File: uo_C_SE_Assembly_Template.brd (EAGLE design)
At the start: 40 x 110.5 mm, 0 parts

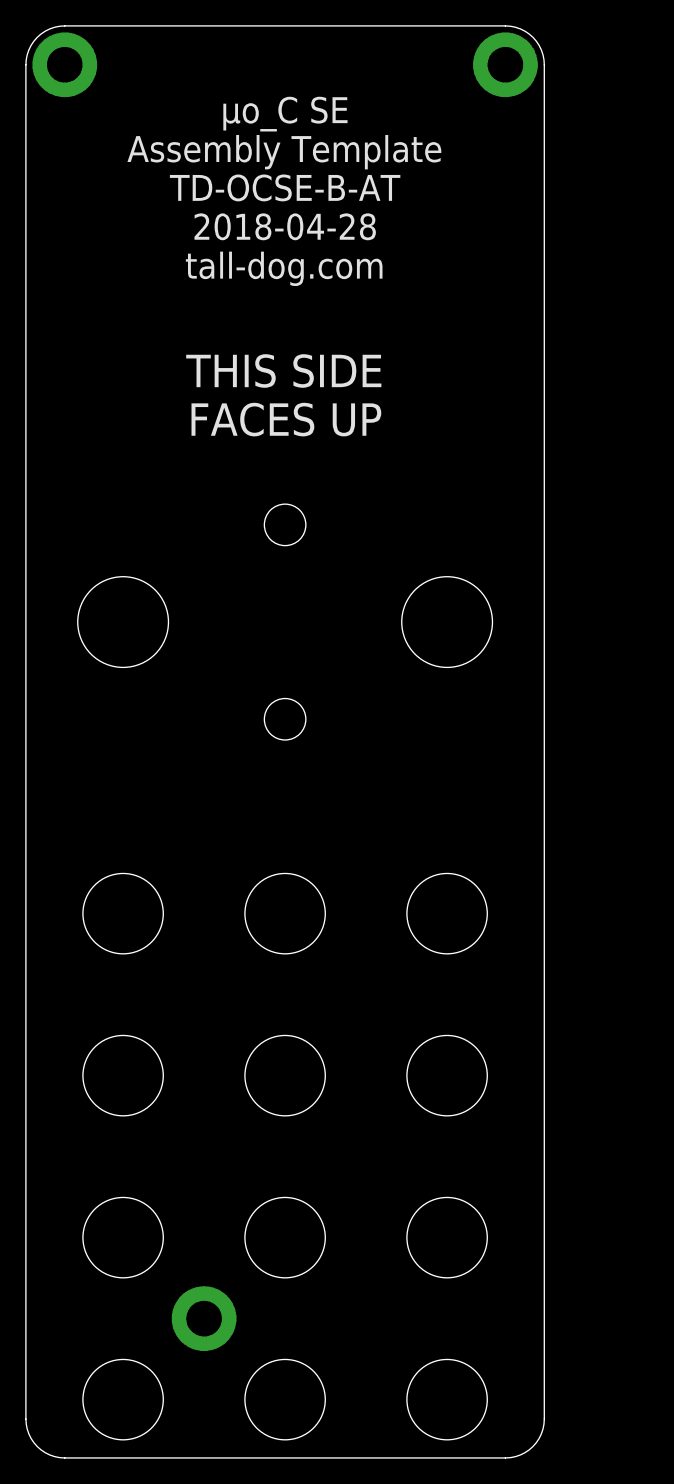
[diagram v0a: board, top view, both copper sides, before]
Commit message: assembly process updates
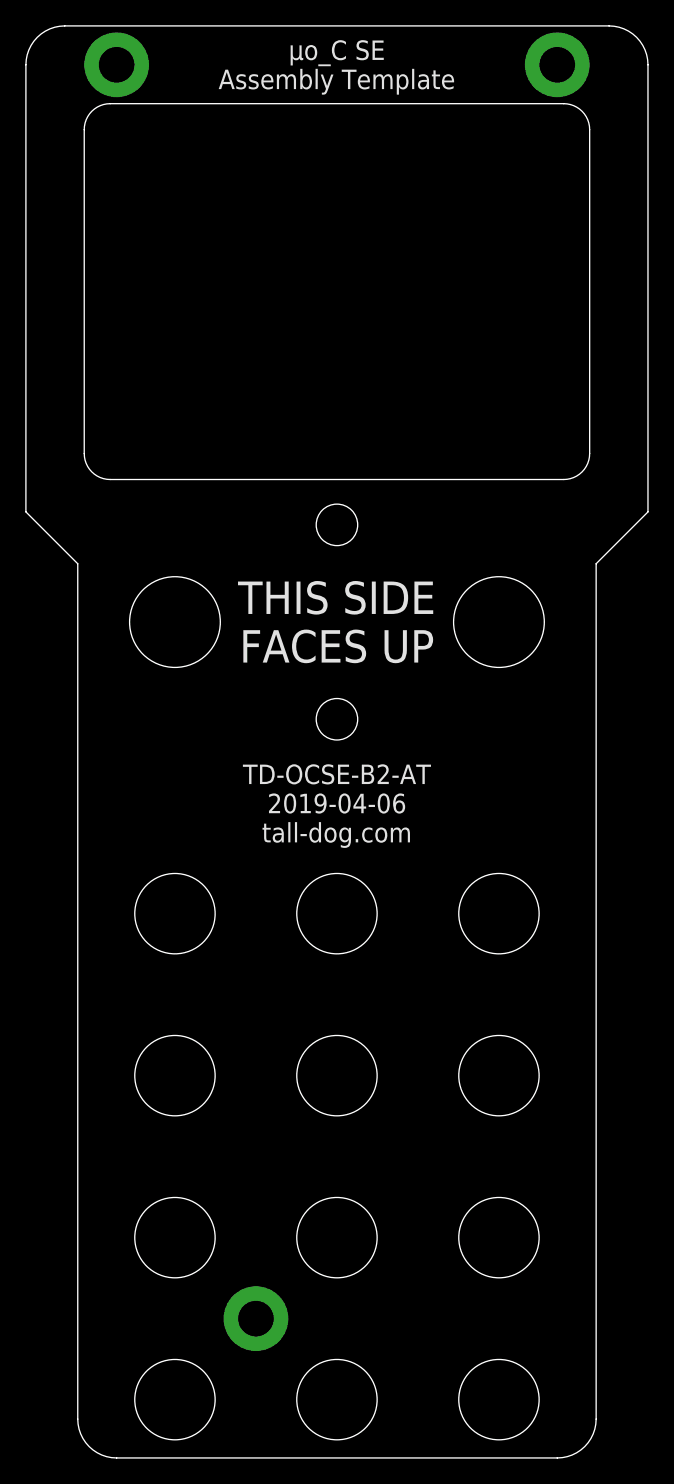
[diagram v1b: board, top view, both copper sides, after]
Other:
- board size 40 x 110.5 mm -> 48 x 110.5 mm
- board text added: "TD-OCSE-B2-AT 2019-04-06 tall-dog.com"
- board text added: "µo_C SE Assembly Template"
- board text removed: "µo_C SE Assembly Template TD-OCSE-B-AT 2018-04-28 tall-dog.com"
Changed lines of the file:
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@@
 <?xml version="1.0" encoding="utf-8"?>
 <!DOCTYPE eagle SYSTEM "eagle.dtd">
-<eagle version="9.0.0">
+<eagle version="9.3.1">
 <drawing>
 <settings>
@@
 <setting verticaltext="up"/>
 </settings>
-<grid distance="1" unitdist="mm" unit="mm" style="lines" multiple="1" display="yes" altdistance="0.1" altunitdist="mm" altunit="mm"/>
+<grid distance="4" unitdist="mm" unit="mm" style="lines" multiple="1" display="yes" altdistance="0.1" altunitdist="mm" altunit="mm"/>
 <layers>
 <layer number="1" name="Top" color="4" fill="1" visible="yes" active="yes"/>
-<layer number="2" name="Route2" color="1" fill="3" visible="no" active="no"/>
-<layer number="15" name="Route15" color="4" fill="6" visible="no" active="no"/>
 <layer number="16" name="Bottom" color="1" fill="1" visible="yes" active="yes"/>
 <layer number="17" name="Pads" color="2" fill="1" visible="yes" active="yes"/>
@@
 <board>
 <plain>
-<wire x1="3" y1="0" x2="37" y2="0" width="0" layer="20"/>
-<wire x1="40" y1="3" x2="40" y2="107.5" width="0" layer="20"/>
-<wire x1="37" y1="110.5" x2="3" y2="110.5" width="0" layer="20"/>
-<wire x1="0" y1="107.5" x2="0" y2="3" width="0" layer="20"/>
+<wire x1="7" y1="0" x2="41" y2="0" width="0" layer="20"/>
+<wire x1="44" y1="3" x2="44" y2="69" width="0" layer="20"/>
+<wire x1="44" y1="69" x2="48" y2="73" width="0" layer="20"/>
+<wire x1="48" y1="73" x2="48" y2="107.5" width="0" layer="20"/>
+<wire x1="45" y1="110.5" x2="3" y2="110.5" width="0" layer="20"/>
+<wire x1="0" y1="107.5" x2="0" y2="73" width="0" layer="20"/>
+<wire x1="0" y1="73" x2="4" y2="69" width="0" layer="20"/>
+<wire x1="4" y1="69" x2="4" y2="3" width="0" layer="20"/>
 <wire x1="0" y1="107.5" x2="3" y2="110.5" width="0" layer="20" curve="-90"/>
-<wire x1="3" y1="0" x2="0" y2="3" width="0" layer="20" curve="-90"/>
-<wire x1="40" y1="3" x2="37" y2="0" width="0" layer="20" curve="-90"/>
-<wire x1="37" y1="110.5" x2="40" y2="107.5" width="0" layer="20" curve="-90"/>
-<hole x="7.5" y="64.5" drill="7"/>
-<hole x="32.5" y="64.5" drill="7"/>
-<hole x="20" y="72" drill="3.2"/>
-<hole x="20" y="57" drill="3.2"/>
-<hole x="7.5" y="42" drill="6.2"/>
-<hole x="20" y="42" drill="6.2"/>
-<hole x="32.5" y="42" drill="6.2"/>
-<hole x="20" y="29.5" drill="6.2"/>
-<hole x="7.5" y="29.5" drill="6.2"/>
-<hole x="32.5" y="29.5" drill="6.2"/>
-<hole x="32.5" y="17" drill="6.2"/>
-<hole x="20" y="17" drill="6.2"/>
-<hole x="7.5" y="17" drill="6.2"/>
-<hole x="7.5" y="4.5" drill="6.2"/>
-<hole x="20" y="4.5" drill="6.2"/>
-<hole x="32.5" y="4.5" drill="6.2"/>
-<text x="20" y="98" size="2" layer="21" align="center">µo_C SE
-Assembly Template
-TD-OCSE-B-AT
-2018-04-28
+<wire x1="7" y1="0" x2="4" y2="3" width="0" layer="20" curve="-90"/>
+<wire x1="44" y1="3" x2="41" y2="0" width="0" layer="20" curve="-90"/>
+<wire x1="45" y1="110.5" x2="48" y2="107.5" width="0" layer="20" curve="-90"/>
+<hole x="11.5" y="64.5" drill="7"/>
+<hole x="36.5" y="64.5" drill="7"/>
+<hole x="24" y="72" drill="3.2"/>
+<hole x="24" y="57" drill="3.2"/>
+<hole x="11.5" y="42" drill="6.2"/>
+<hole x="24" y="42" drill="6.2"/>
+<hole x="36.5" y="42" drill="6.2"/>
+<hole x="24" y="29.5" drill="6.2"/>
+<hole x="11.5" y="29.5" drill="6.2"/>
+<hole x="36.5" y="29.5" drill="6.2"/>
+<hole x="36.5" y="17" drill="6.2"/>
+<hole x="24" y="17" drill="6.2"/>
+<hole x="11.5" y="17" drill="6.2"/>
+<hole x="11.5" y="4.5" drill="6.2"/>
+<hole x="24" y="4.5" drill="6.2"/>
+<hole x="36.5" y="4.5" drill="6.2"/>
+<text x="24" y="107.5" size="1.5" layer="21" ratio="10" align="center">µo_C SE
+Assembly Template</text>
+<text x="24" y="64.5" size="2.5" layer="21" ratio="10" rot="R180" align="center">THIS SIDE
+FACES UP</text>
+<text x="24" y="64.5" size="2" layer="22" ratio="10" rot="MR180" align="center">THIS SIDE
+FACES DOWN</text>
+<text x="24" y="50.5" size="1.5" layer="21" ratio="10" align="center">TD-OCSE-B2-AT
+2019-04-06
 tall-dog.com</text>
-<text x="20" y="82" size="2.5" layer="21" ratio="10" rot="R180" align="center">THIS SIDE
-FACES UP</text>
-<text x="20" y="82" size="2.5" layer="22" ratio="10" rot="MR180" align="center">THIS SIDE
-FACES DOWN</text>
-<text x="20" y="98" size="2" layer="22" rot="MR0" align="center">µo_C SE
-Assembly Template
-TD-OCSE-B-AT
-2018-04-28
+<text x="24" y="107.5" size="1.5" layer="22" ratio="10" rot="MR0" align="center">µo_C SE
+Assembly Template</text>
+<text x="24" y="50.5" size="1.5" layer="22" ratio="10" rot="MR0" align="center">TD-OCSE-B2-AT
+2019-04-06
 tall-dog.com</text>
+<wire x1="6.5" y1="104.5" x2="41.5" y2="104.5" width="0" layer="20"/>
+<wire x1="43.5" y1="102.5" x2="43.5" y2="77.5" width="0" layer="20"/>
+<wire x1="41.5" y1="75.5" x2="6.5" y2="75.5" width="0" layer="20"/>
+<wire x1="4.5" y1="77.5" x2="4.5" y2="102.5" width="0" layer="20"/>
+<wire x1="6.5" y1="75.5" x2="4.5" y2="77.5" width="0" layer="20" curve="-90"/>
+<wire x1="4.5" y1="102.5" x2="6.5" y2="104.5" width="0" layer="20" curve="-90"/>
+<wire x1="41.5" y1="104.5" x2="43.5" y2="102.5" width="0" layer="20" curve="-90"/>
+<wire x1="43.5" y1="77.5" x2="41.5" y2="75.5" width="0" layer="20" curve="-90"/>
 </plain>
 <attributes>
@@
 <param name="checkStop" value="1"/>
 <param name="checkValues" value="0"/>
+<param name="checkNames" value="1"/>
+<param name="checkWireStubs" value="1"/>
+<param name="checkPolygonWidth" value="0"/>
 <param name="useDiameter" value="13"/>
 <param name="maxErrors" value="50"/>
@@
 <signals>
 <signal name="S$1">
-<via x="3" y="107.5" extent="1-16" drill="2.75" diameter="5"/>
+<via x="7" y="107.5" extent="1-16" drill="2.75" diameter="5"/>
 </signal>
 <signal name="S$2">
-<via x="37" y="107.5" extent="1-16" drill="2.75" diameter="5"/>
+<via x="41" y="107.5" extent="1-16" drill="2.75" diameter="5"/>
 </signal>
 <signal name="S$3">
-<via x="13.75" y="10.75" extent="1-16" drill="2.75" diameter="5"/>
+<via x="17.75" y="10.75" extent="1-16" drill="2.75" diameter="5"/>
 </signal>
 </signals>
+<mfgpreviewcolors>
+<mfgpreviewcolor name="soldermaskcolor" color="0xC8008000"/>
+<mfgpreviewcolor name="silkscreencolor" color="0xFFFEFEFE"/>
+<mfgpreviewcolor name="backgroundcolor" color="0xFF282828"/>
+<mfgpreviewcolor name="coppercolor" color="0xFFFFBF00"/>
+<mfgpreviewcolor name="substratecolor" color="0xFF786E46"/>
+</mfgpreviewcolors>
 <errors>
 </errors>
